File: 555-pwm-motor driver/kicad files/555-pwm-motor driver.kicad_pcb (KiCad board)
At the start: 2 copper layers, 19 parts, among them J1 Screw_Terminal_01x02, J2 Screw_Terminal_01x02, J3 Conn_01x01_Male, J4 Conn_01x01_Male, Q1 IRLZ44N, U1 LM7805_TO220, U2 SE555P, U3 3PIN-POT-LOCAL

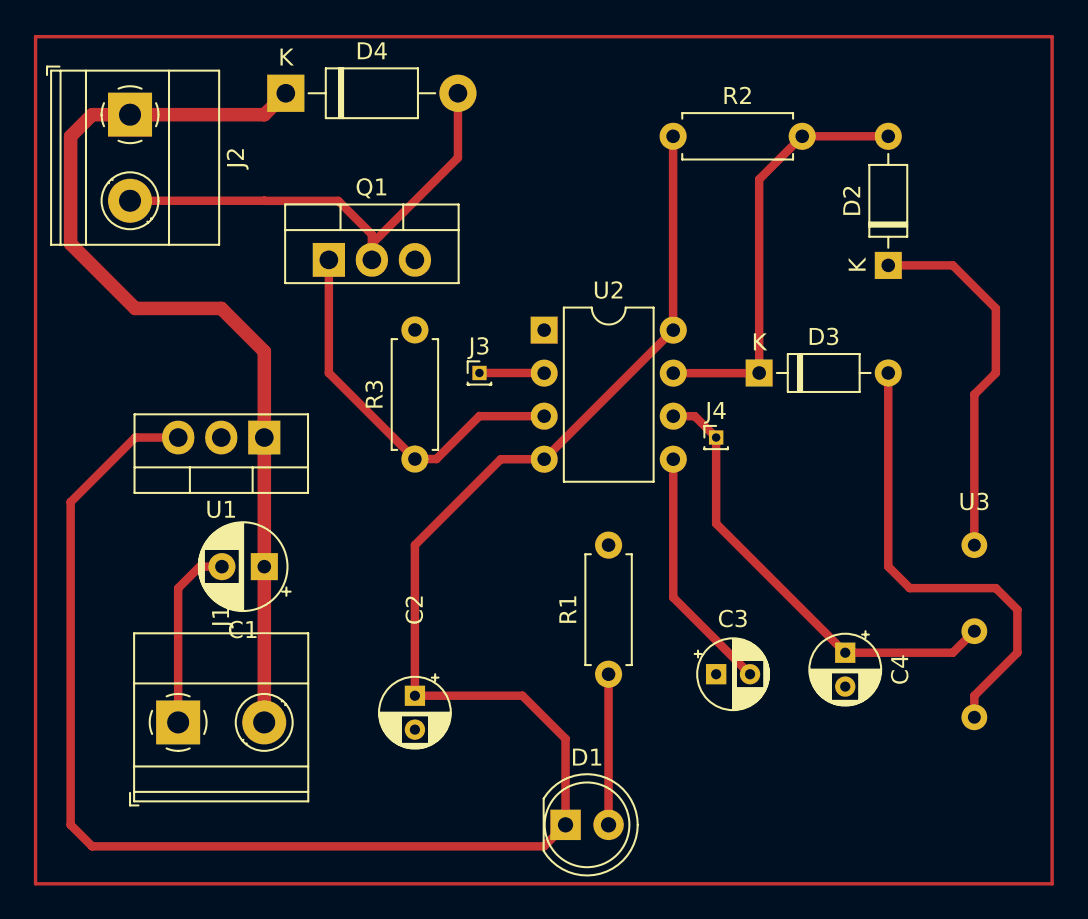
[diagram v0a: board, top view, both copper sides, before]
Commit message: Cleaning up pcb
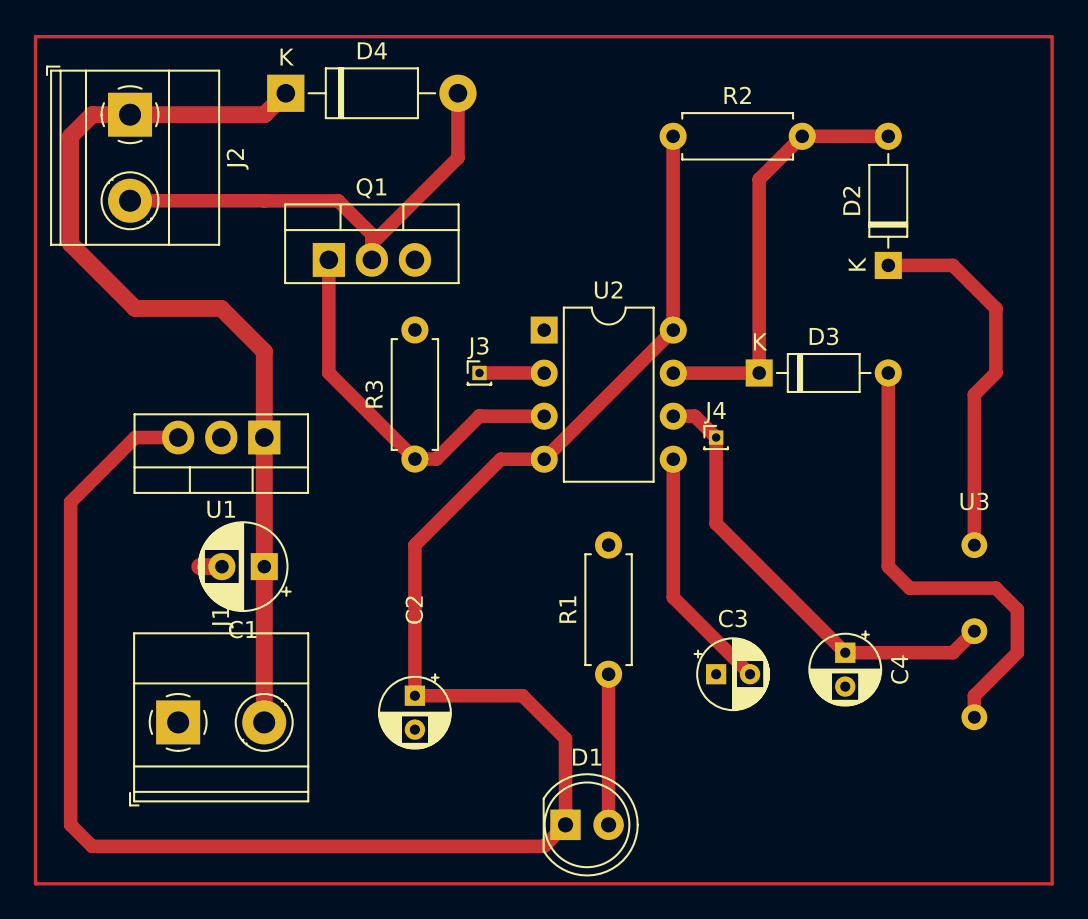
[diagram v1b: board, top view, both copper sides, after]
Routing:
- net GND: track 11.1 -> 1.31 mm
